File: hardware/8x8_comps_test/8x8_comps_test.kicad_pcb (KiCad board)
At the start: 2 copper layers, 77.5 x 45.7 mm, 24 parts

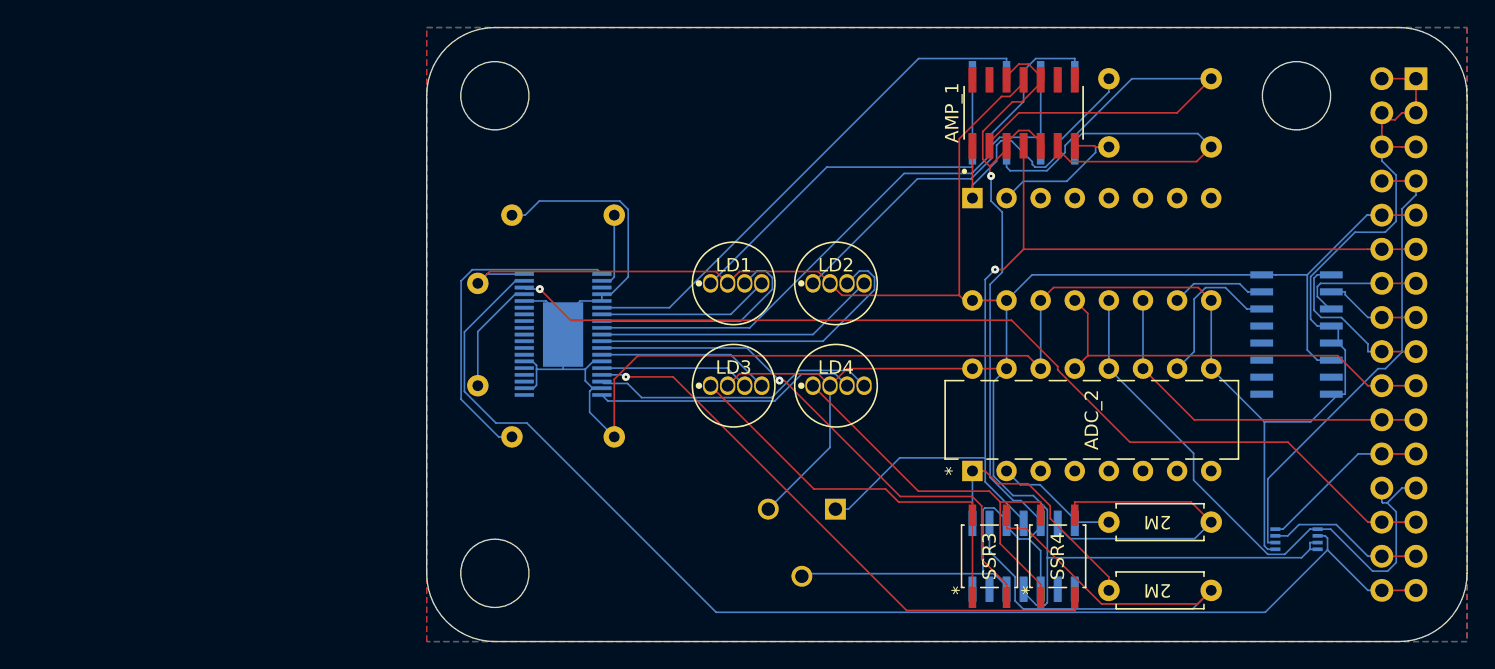
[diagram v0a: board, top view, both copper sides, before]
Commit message: Updated PCB
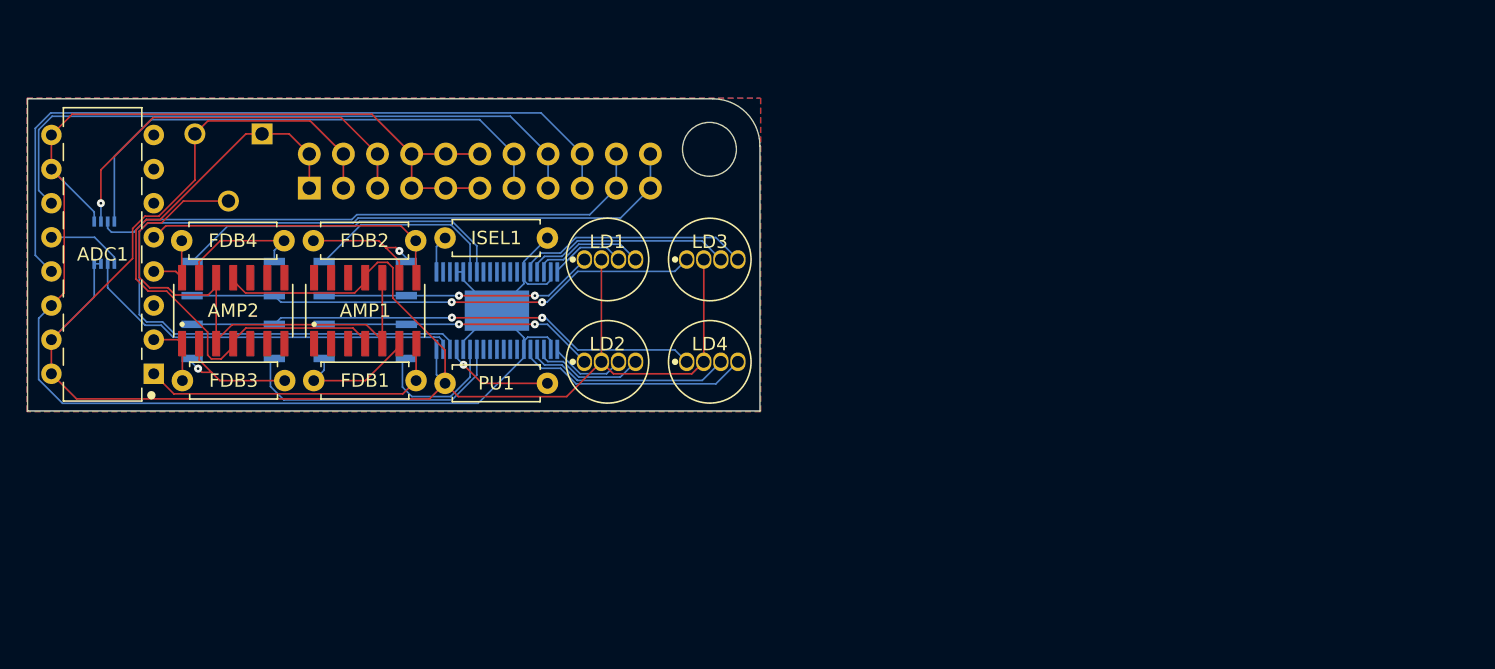
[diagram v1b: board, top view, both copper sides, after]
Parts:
- removed ADC_1, ADC_2: MCP3008-I/P-DIP16, ADC:MCP3008-I&slash_P
- removed AMP_1, AMP_2: MCP619-I/SL, Op-Amp:footprints
- removed Addr_Sel_1: 100K, Resistor_THT:R_Axial_DIN0207_L6.3mm_D2.5mm_P7.62mm_Horizontal
- removed Amp_Fdbk_1, Amp_Fdbk_2, Amp_Fdbk_3, Amp_Fdbk_4: 2M, Resistor_THT:R_Axial_DIN0207_L6.3mm_D2.5mm_P7.62mm_Horizontal
- removed DEMUX_1: 74HC138D-Q100,118, DEMUX:footprints
- removed Drv_I_Sel_1: 2K, Resistor_THT:R_Axial_DIN0207_L6.3mm_D2.5mm_P7.62mm_Horizontal
- removed Drv_RST_PU_1: 10K, Resistor_THT:R_Axial_DIN0207_L6.3mm_D2.5mm_P7.62mm_Horizontal
- removed LED_Driver_1: PCA9956BTWY, LED Driver:SOP50P640X110-39N
- removed Lvl_Sftr_1: LSF0102DCH, Level Shifter:LSF0102DCH
- removed Pin_Header_1: Conn_02x16_Odd_Even, Connector_PinHeader_2.54mm:PinHeader_2x16_P2.54mm_Vertical
- removed Rev_Bias_Sel_1: 100K, Potentiometer_THT:Potentiometer_Runtron_RM-065_Vertical
- added ADC1: MCP3008-I/P-DIP16, ADC:MCP3008-I&slash_P, F.Cu at (72.4, 84.2)
- added AMP1: MCP619-I/SL, Op-Amp:footprints, F.Cu at (91.9, 88.4)
- added AMP2: MCP619-I/SL, Op-Amp:footprints, F.Cu at (82.1, 88.4)
- added DRV1: PCA9956BTWY, LED Driver:SOP50P640X110-39N, B.Cu at (101.8, 88.4)
- added FDB1: 2M, Resistor - Through-Hole:footprints, F.Cu at (91.9, 93.6)
- added FDB2: 2M, Resistor - Through-Hole:footprints, F.Cu at (91.9, 83.2)
- added FDB3: 2M, Resistor - Through-Hole:footprints, F.Cu at (82.1, 93.6)
- added FDB4: 2M, Resistor - Through-Hole:footprints, F.Cu at (82.1, 83.2)
- added ISEL1: 2K, Resistor - Through-Hole:footprints, F.Cu at (101.7, 83.0)
- added PH1: Conn_02x11_Odd_Even, Connector_PinSocket_2.54mm:PinSocket_2x11_P2.54mm_Vertical, B.Cu at (87.8, 79.3)
- added PU1: 10K, Resistor - Through-Hole:footprints, F.Cu at (101.7, 93.8)
- added RBSEL1: 100K, Potentiometer_THT:Potentiometer_Runtron_RM-065_Vertical, B.Cu at (84.3, 75.2)
- added SFTR1: VSSOP8_SOT765-1_NEX, Level Shifter:LSF0102DCH, B.Cu at (72.5, 83.3)
- SSR3, SSR4: moved to B.Cu
- moved SSR4 63.4 mm to (82.1, 90.7), turned to 180 degrees
- moved SSR3 60.0 mm to (82.1, 86.0), turned to 0 degrees
- moved SSR2 54.3 mm to (91.9, 90.7), turned to 180 degrees
- moved SSR1 48.1 mm to (91.9, 86.0), turned to 0 degrees
- moved LD2 18.0 mm to (110.0, 92.2)
- moved LD3 9.56 mm to (117.6, 84.6)
- moved LD1 9.56 mm to (110.0, 84.6)
- moved LD4 9.56 mm to (117.6, 92.2)
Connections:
- net /LED Row IO 1/LDRow/LD1_R renamed /LDRow/LD1_R
- net /LED Row IO 1/LDRow/LD2_R renamed /LDRow/LD2_R
- net /LED Row IO 2/LDRow/LD1_R renamed /LDRow1/LD1_R
- net /LED Row IO 2/LDRow/LD2_R renamed /LDRow1/LD2_R
- LD1 pad 3: /LED Row IO 1/LD1_TX_B -> /LDRow/LD1_B
- LD1 pad 4: /LED Row IO 1/LD1_TX_G -> /LDRow/LD1_G
- LD2 pad 3: /LED Row IO 1/LD2_TX_B -> /LDRow/LD2_B
- LD2 pad 4: /LED Row IO 1/LD2_TX_G -> /LDRow/LD2_G
- LD3 pad 3: /LED Row IO 2/LD1_TX_B -> /LDRow1/LD1_B
- LD3 pad 4: /LED Row IO 2/LD1_TX_G -> /LDRow1/LD1_G
- LD4 pad 3: /LED Row IO 2/LD2_TX_B -> /LDRow1/LD2_B
- LD4 pad 4: /LED Row IO 2/LD2_TX_G -> /LDRow1/LD2_G
- SSR1 pad 2: /LED Row IO 1/LD1_TX_R -> Net-(DRV1-Pad6)
- SSR1 pad 3: /LED Row IO 1/ LDRow_Amps/Amp_IP_1 -> Net-(AMP1-Pad9)
- SSR2 pad 2: /LED Row IO 1/LD2_TX_R -> Net-(DRV1-Pad33)
- SSR2 pad 3: /LED Row IO 1/ LDRow_Amps/Amp_IP_2 -> Net-(AMP1-Pad6)
- SSR3 pad 2: /LED Row IO 2/LD1_TX_R -> Net-(DRV1-Pad7)
- SSR3 pad 3: /LED Row IO 2/ LDRow_Amps/Amp_IP_1 -> Net-(AMP2-Pad13)
- SSR4 pad 2: /LED Row IO 2/LD2_TX_R -> Net-(DRV1-Pad32)
- SSR4 pad 3: /LED Row IO 2/ LDRow_Amps/Amp_IP_2 -> Net-(AMP2-Pad2)
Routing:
- net I2C_SDA_5V: track 93.0 -> 29.0 mm
- net +5V: track 186.8 -> 139.6 mm
- net /LED Row IO 1/LD2_TX_R: track 46.7 -> 0.00 mm
- net /LED Row IO 2/LD2_TX_R: track 43.5 -> 0.00 mm, vias 1 -> 0
- net /LED Row IO 2/ LDRow_Amps/Amp_IP_1: track 41.0 -> 0.00 mm
- net /LED Row IO 2/LD1_TX_R: track 40.7 -> 0.00 mm, vias 1 -> 0
- net /LED Row IO 1/LD1_TX_R: track 38.8 -> 0.00 mm
- net SPI_MISO_5V: track 44.5 -> 5.80 mm
- net /LED Row IO 1/ LDRow_Amps/Amp_IP_1: track 38.2 -> 0.00 mm
- net RB Voltage: track 78.8 -> 41.8 mm, vias 1 -> 0
- net GND: track 165.6 -> 130.9 mm
- net I2C_SDA_3V3: track 11.8 -> 42.4 mm
- net +9V: track 72.8 -> 45.1 mm, vias 1 -> 0
- net SPI_MISO_3V3: track 12.8 -> 39.3 mm
- net /LED Row IO 1/LD2_TX_B: track 25.4 -> 0.00 mm
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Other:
- board size 77.5 x 45.7 mm -> 54.5 x 23.2 mm
